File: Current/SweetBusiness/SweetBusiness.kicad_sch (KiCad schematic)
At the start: 57 parts, among them J2 I2C, J4 USB, U0 RP2040, U1 MT2492, U2 W25Q128JVS, U3 USBLC6-2SC6, Y0 CSTCE12M0G55-R0

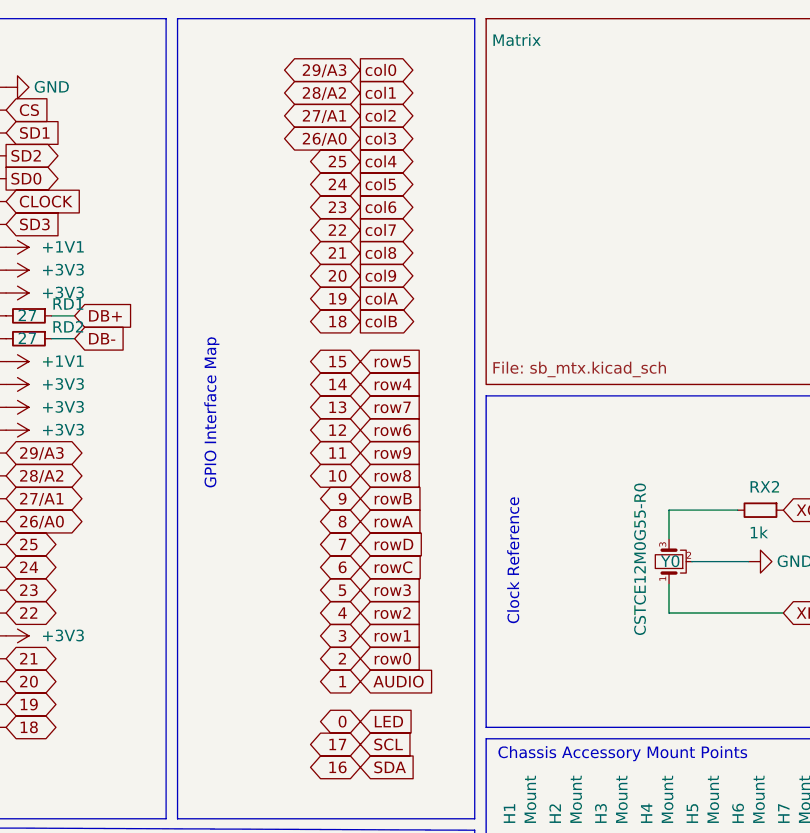
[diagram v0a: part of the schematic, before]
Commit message: Arrow of Time changes, updates to Sweet Business Six
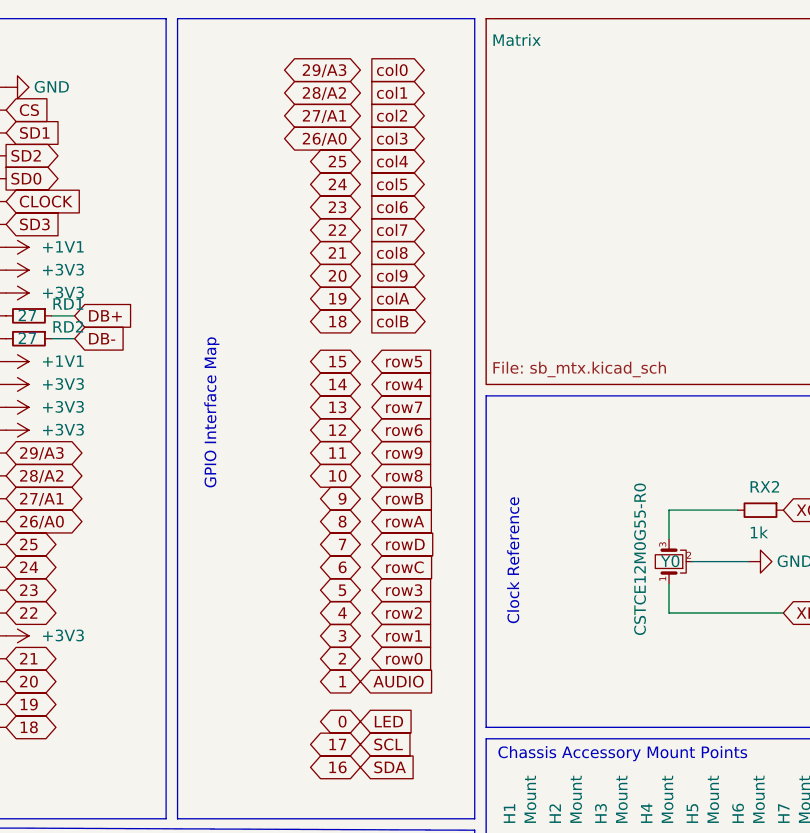
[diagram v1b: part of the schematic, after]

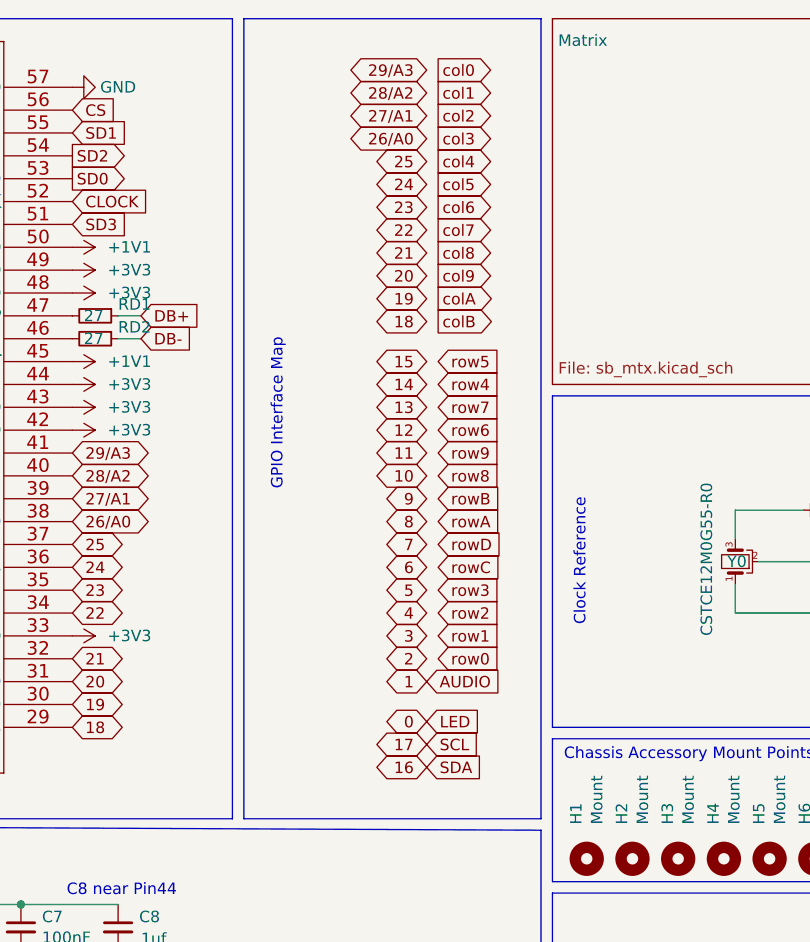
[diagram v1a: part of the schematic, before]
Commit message: Bulk catchup commit 2023-01-21
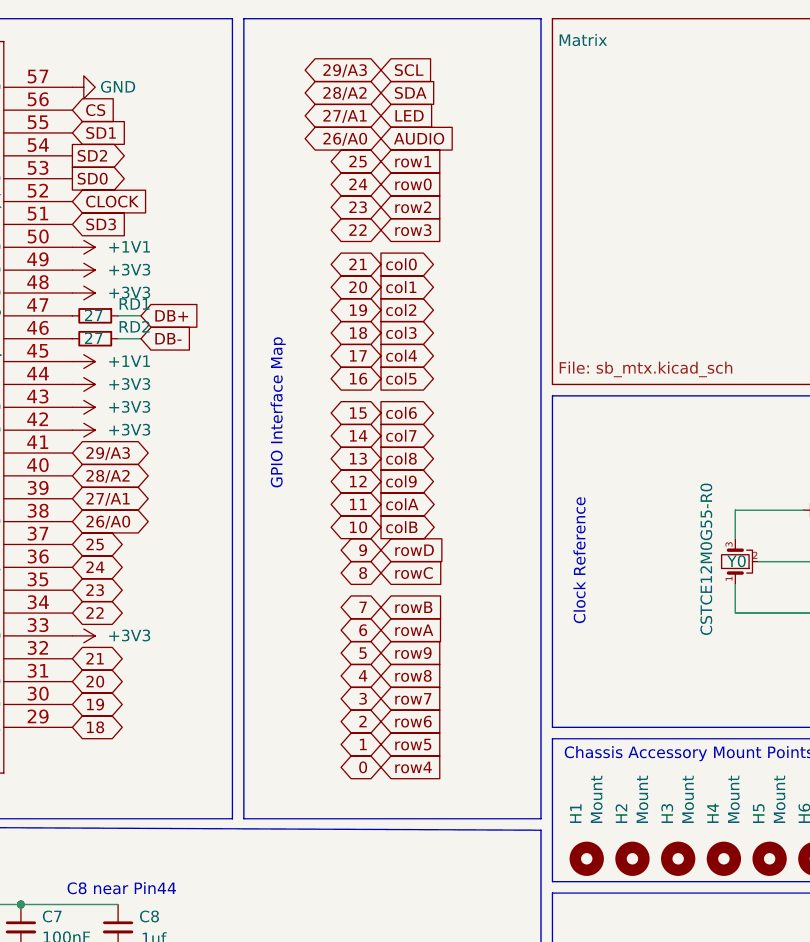
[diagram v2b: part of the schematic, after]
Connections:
- net 1: no longer TX0.1
- net 16: no longer J2.1 (Pin_1)
- net 17: no longer J2.2 (Pin_2)
- net 26/A0: now also TX0.1
- net 28/A2: now also J2.1 (Pin_1)
- net 29/A3: now also J2.2 (Pin_2)

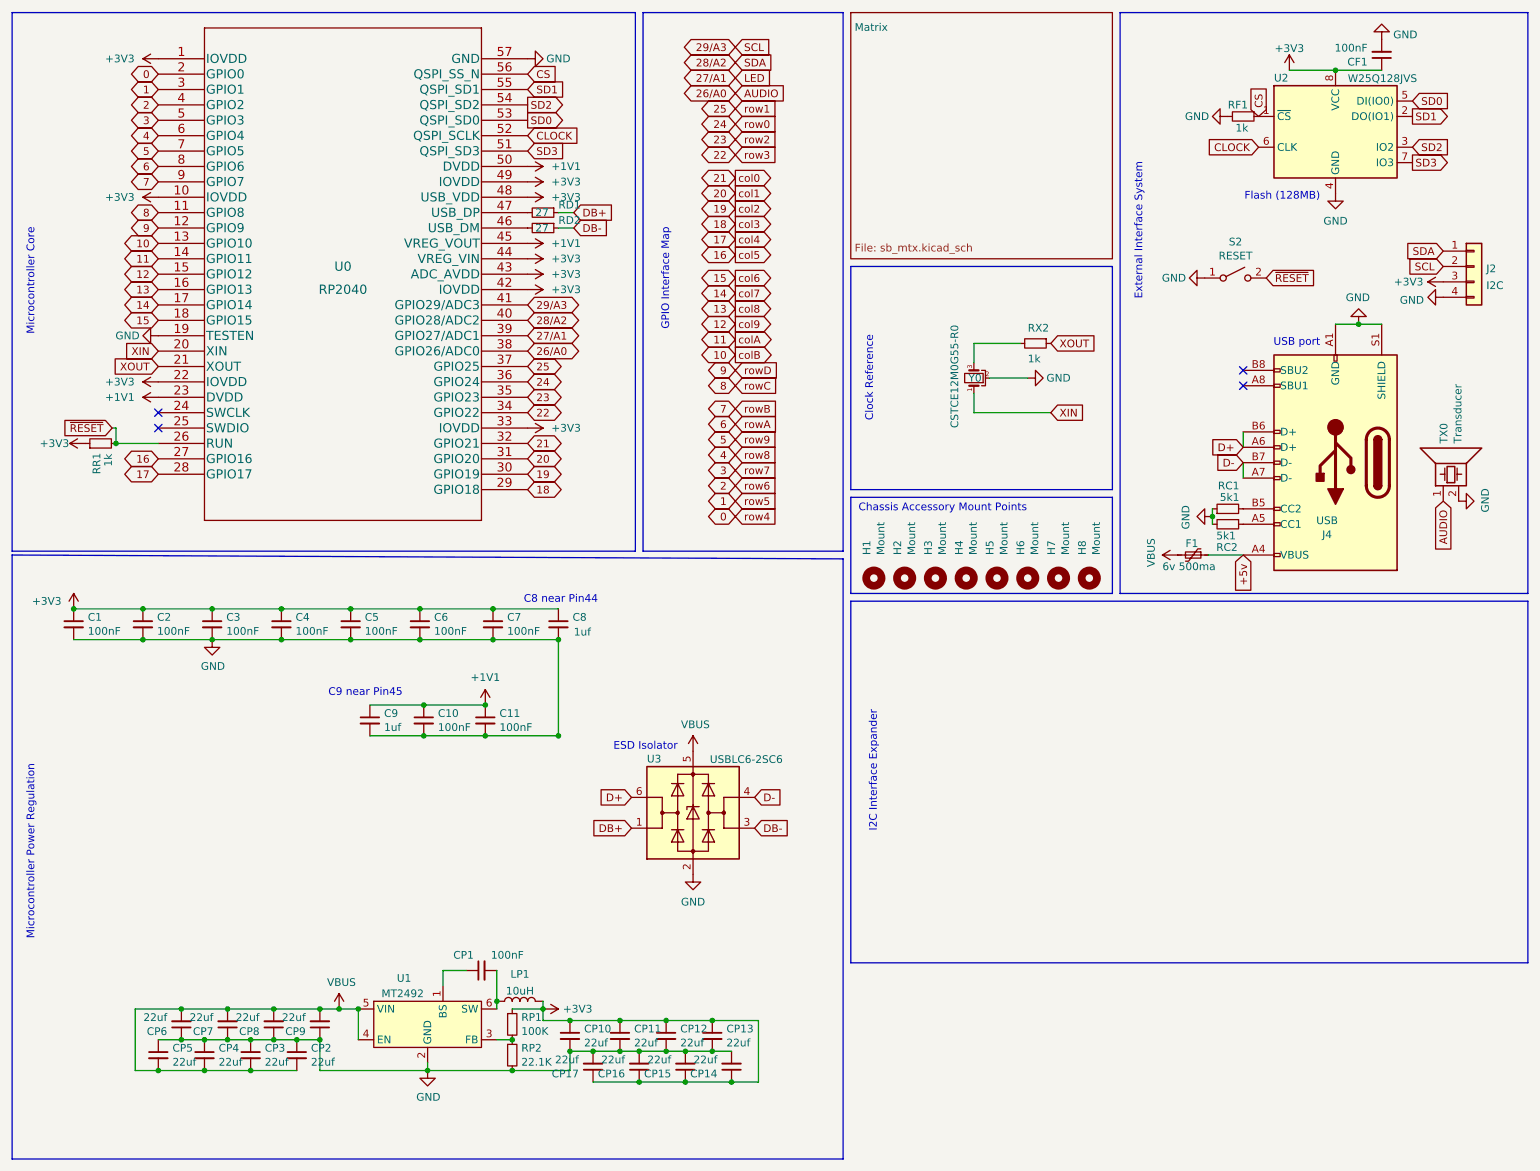
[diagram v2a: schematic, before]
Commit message: oh god there's too much
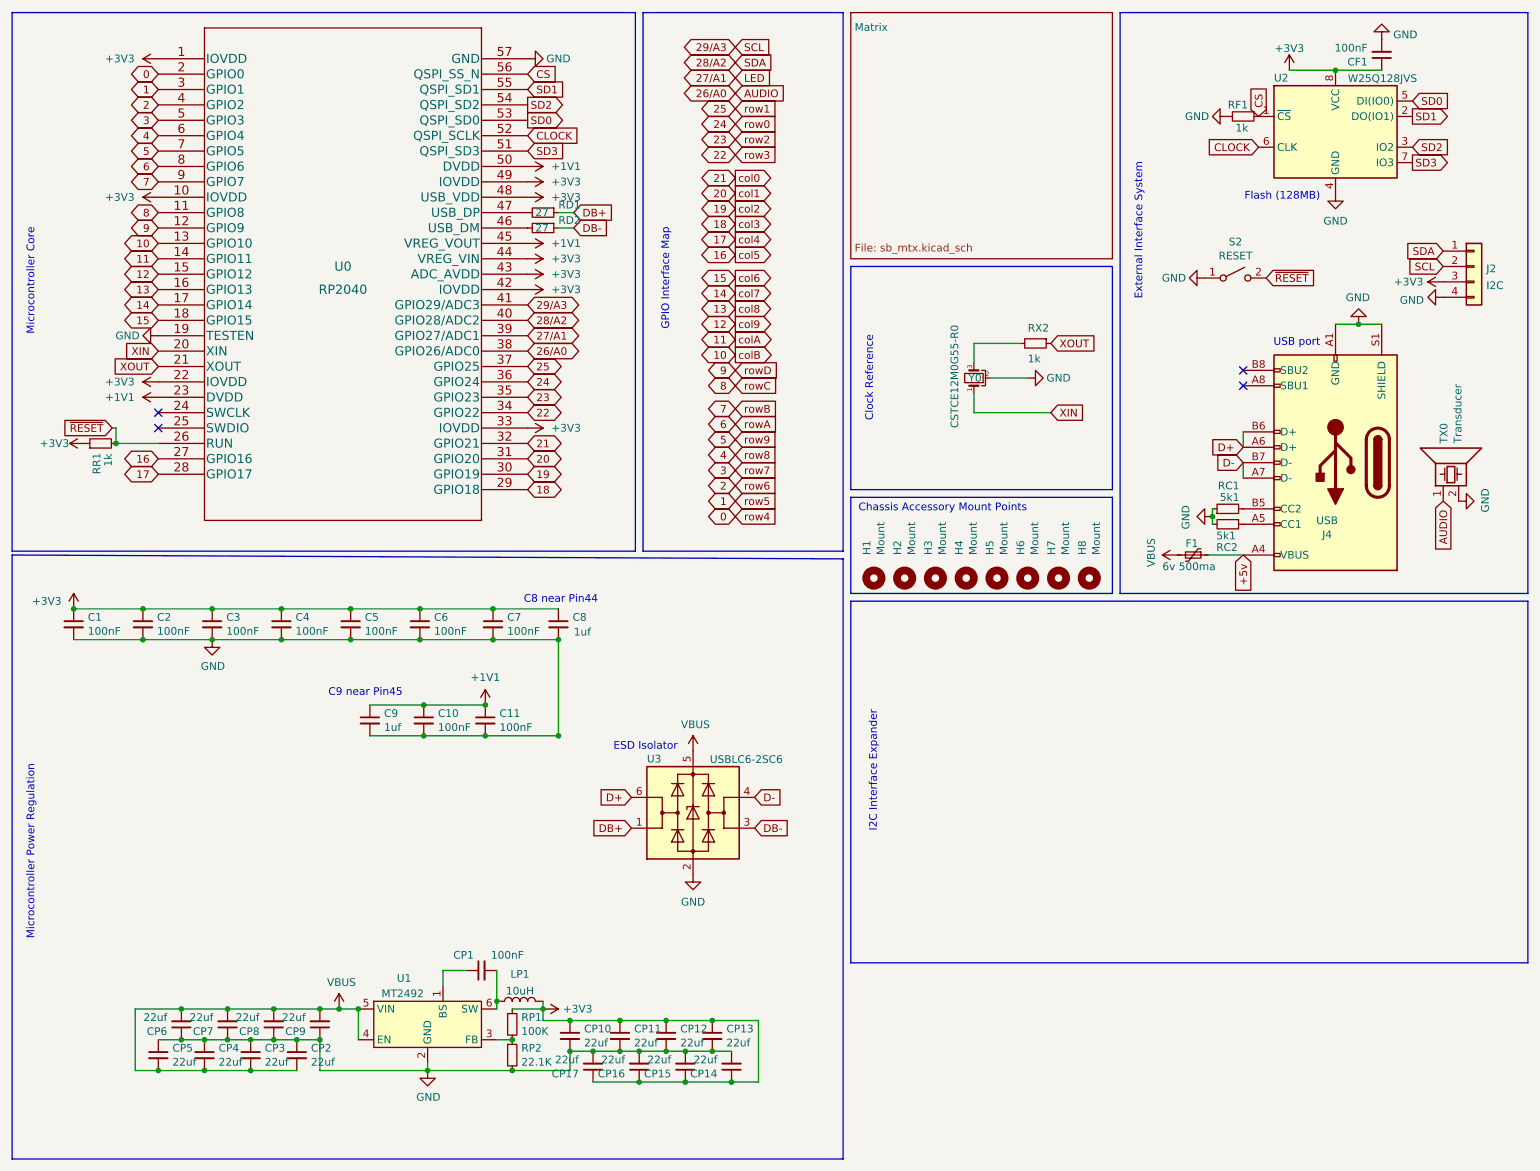
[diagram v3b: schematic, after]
